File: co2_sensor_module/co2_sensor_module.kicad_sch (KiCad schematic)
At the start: 3 parts, among them J2 Conn_01x04, J3 Conn_01x04

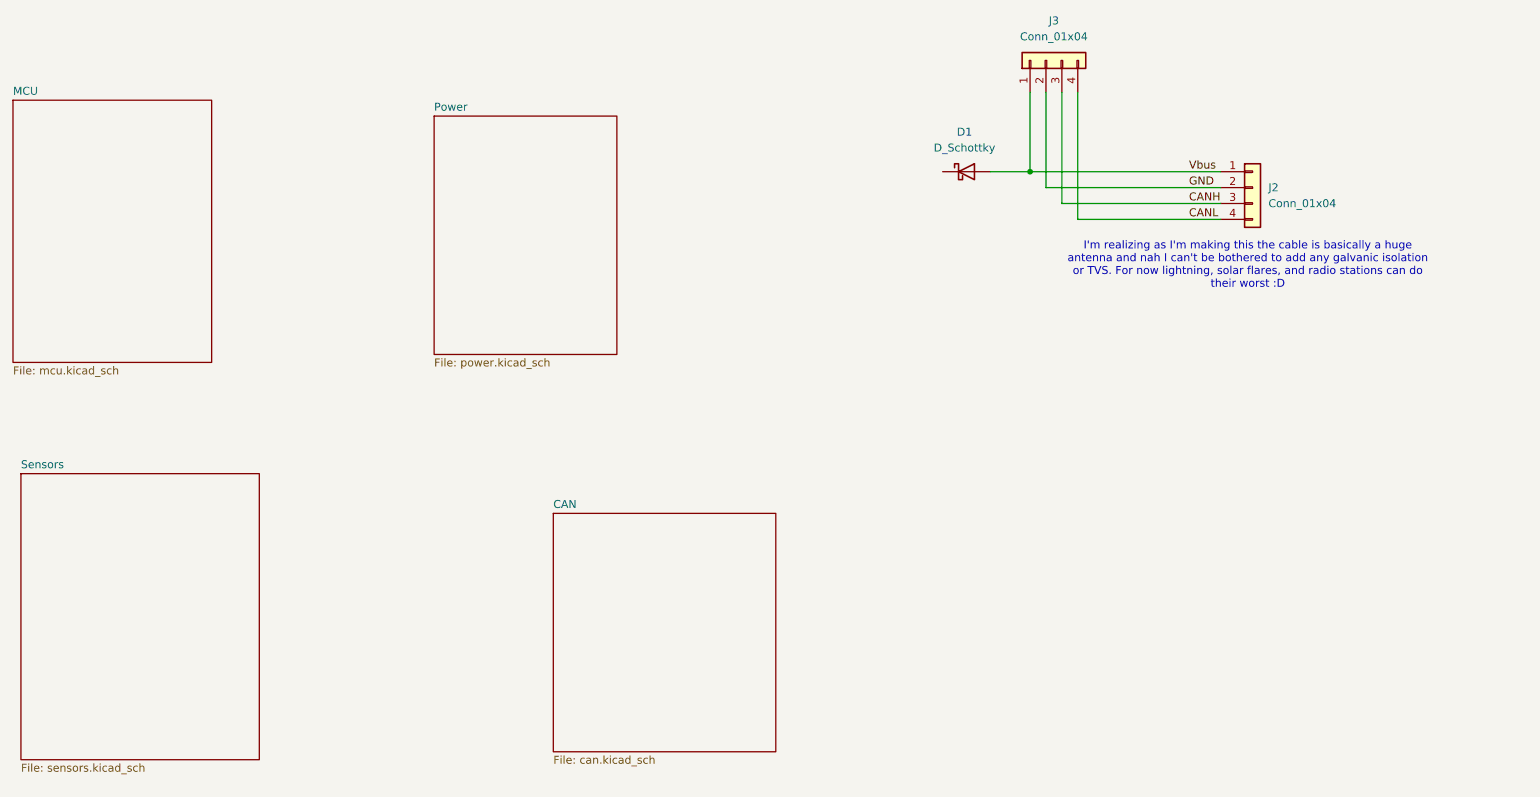
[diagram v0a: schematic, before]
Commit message: first draft of sensor schematic is done!
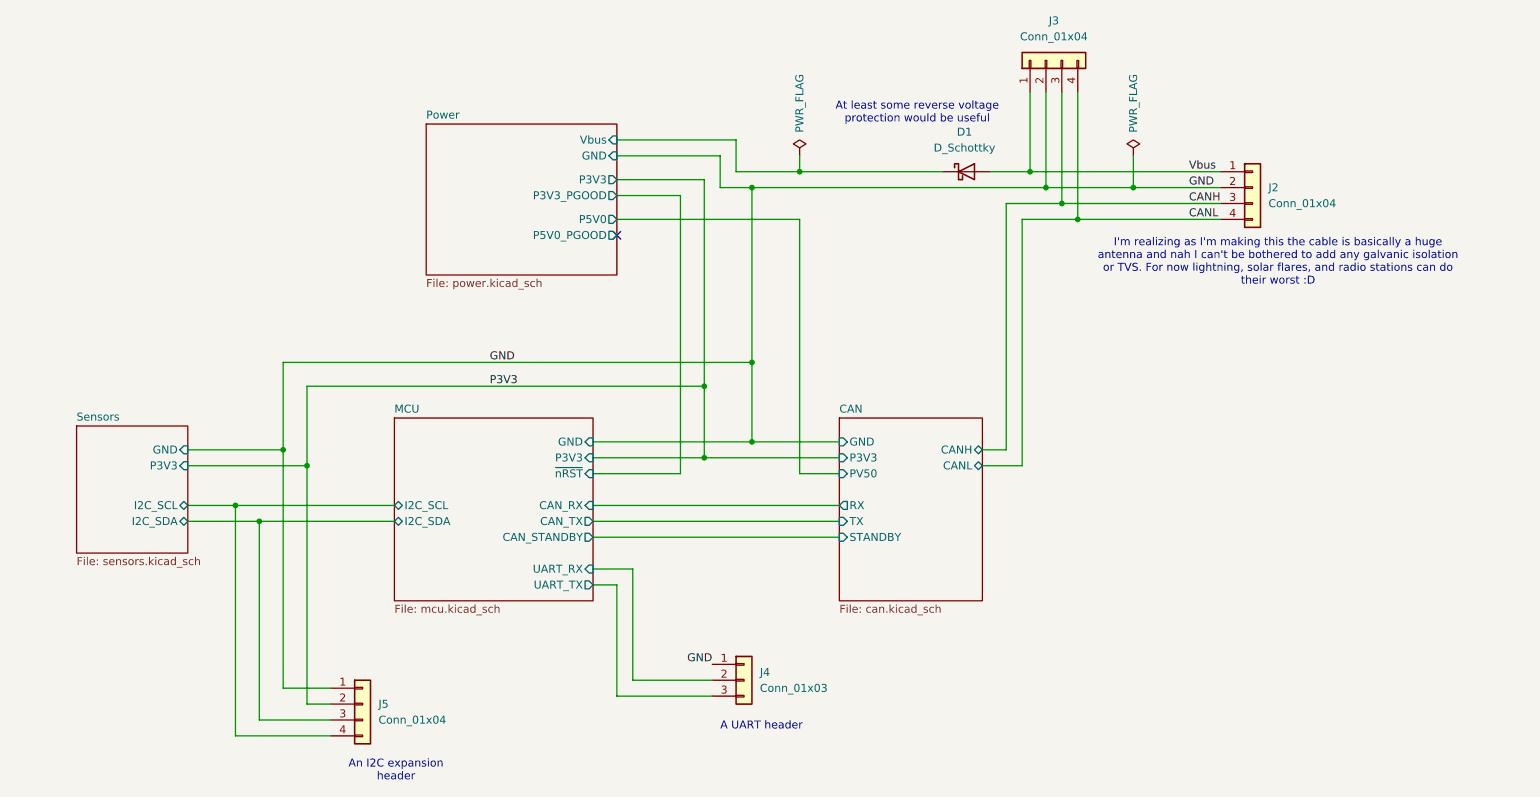
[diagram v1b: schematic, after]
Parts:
- added J4: Conn_01x03, symbol Connector_Generic:Conn_01x03
- added J5: Conn_01x04, symbol Connector_Generic:Conn_01x04
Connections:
- net GND: now also J4.1 (Pin_1), J5.1 (Pin_1)
- net Power/Vbus: now reaches D1.1 (K)
- new net MCU/I2C_SCL: J5.4 (Pin_4)
- new net MCU/I2C_SDA: J5.3 (Pin_3)
- new net MCU/UART_RX: J4.2 (Pin_2)
- new net MCU/UART_TX: J4.3 (Pin_3)
- new net P3V3: J5.2 (Pin_2)
- no-connect marks 0 -> 1
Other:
- sheet CAN ports: added CANH, CANL, GND, P3V3, PV50, RX, STANDBY, TX; removed none
- sheet MCU ports: added CAN_RX, CAN_STANDBY, CAN_TX, GND, I2C_SCL, I2C_SDA, P3V3, UART_RX, UART_TX, ~{nRST}; removed none
- sheet Power ports: added GND, P3V3, P3V3_PGOOD, P5V0, P5V0_PGOOD, Vbus; removed none
- sheet Sensors ports: added GND, I2C_SCL, I2C_SDA, P3V3; removed none
- note added: "A UART header"
- note added: "An I2C expansion header"
- note added: "At least some reverse voltage protection would be useful"
